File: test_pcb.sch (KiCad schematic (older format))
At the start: 22 parts, among them J1 Conn_01x04_Male, J11 Conn_01x20_Female, J8 Conn_01x20_Female, SW1 on/off, SW2 on/off

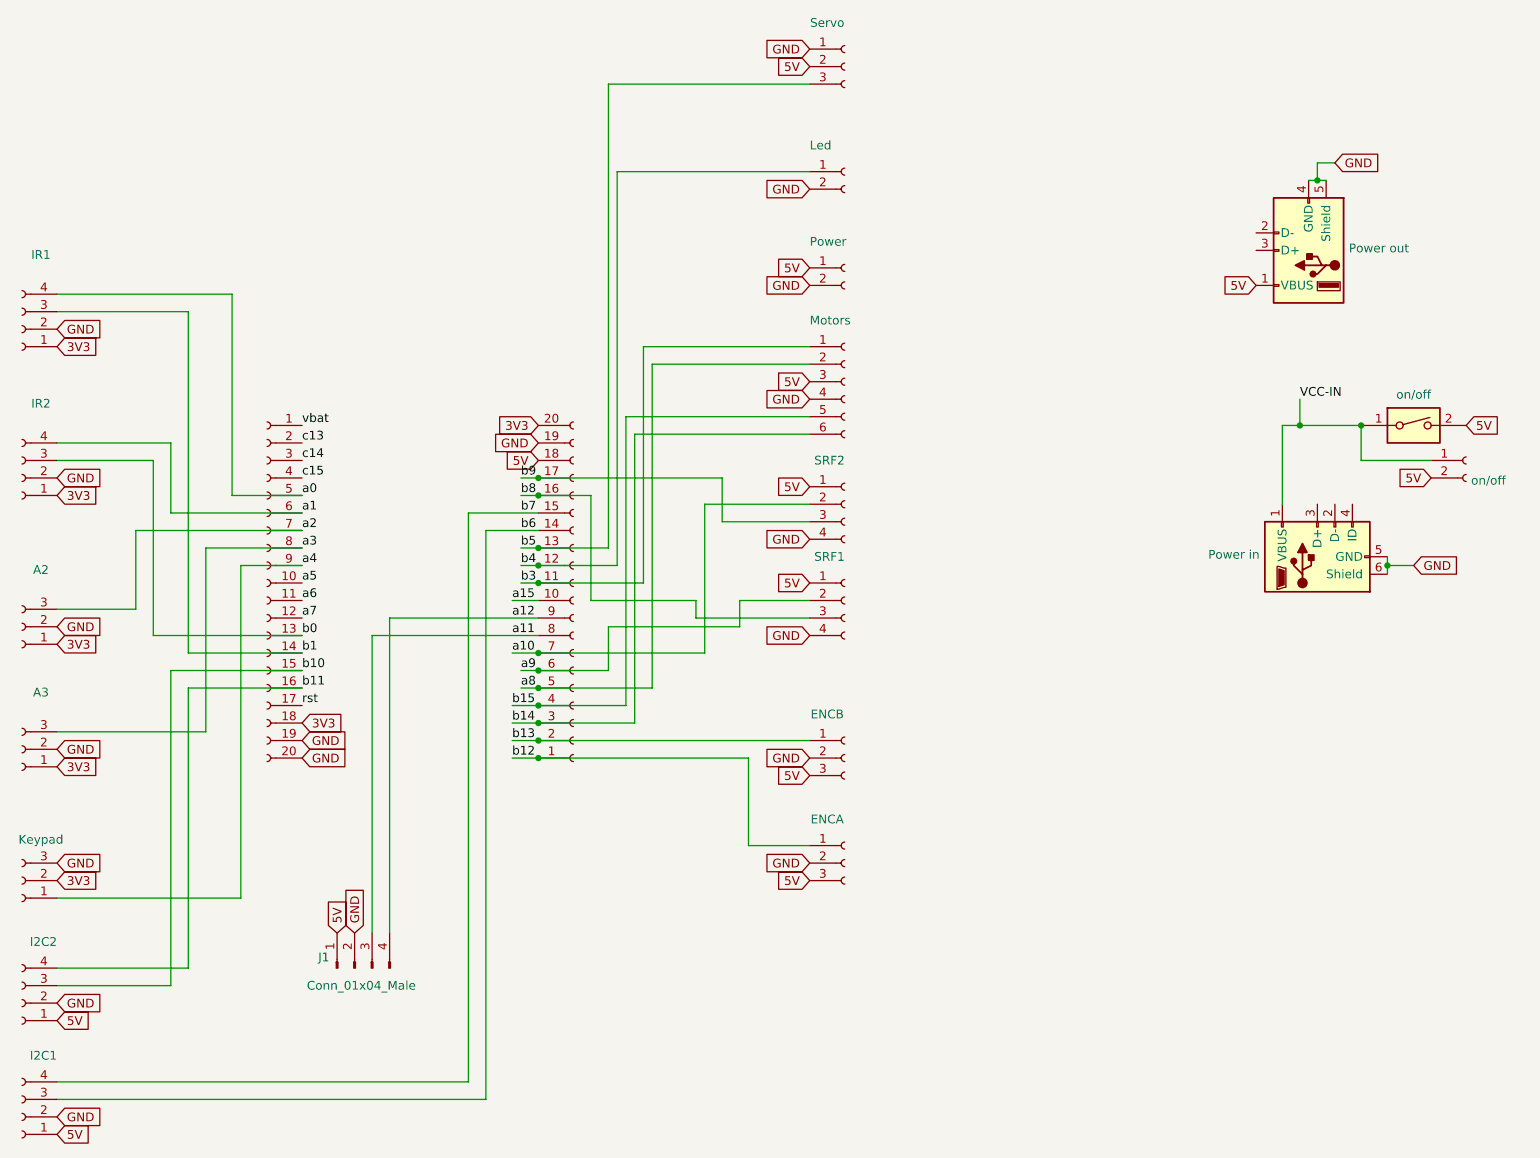
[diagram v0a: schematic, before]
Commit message: changes v2, ugly routing
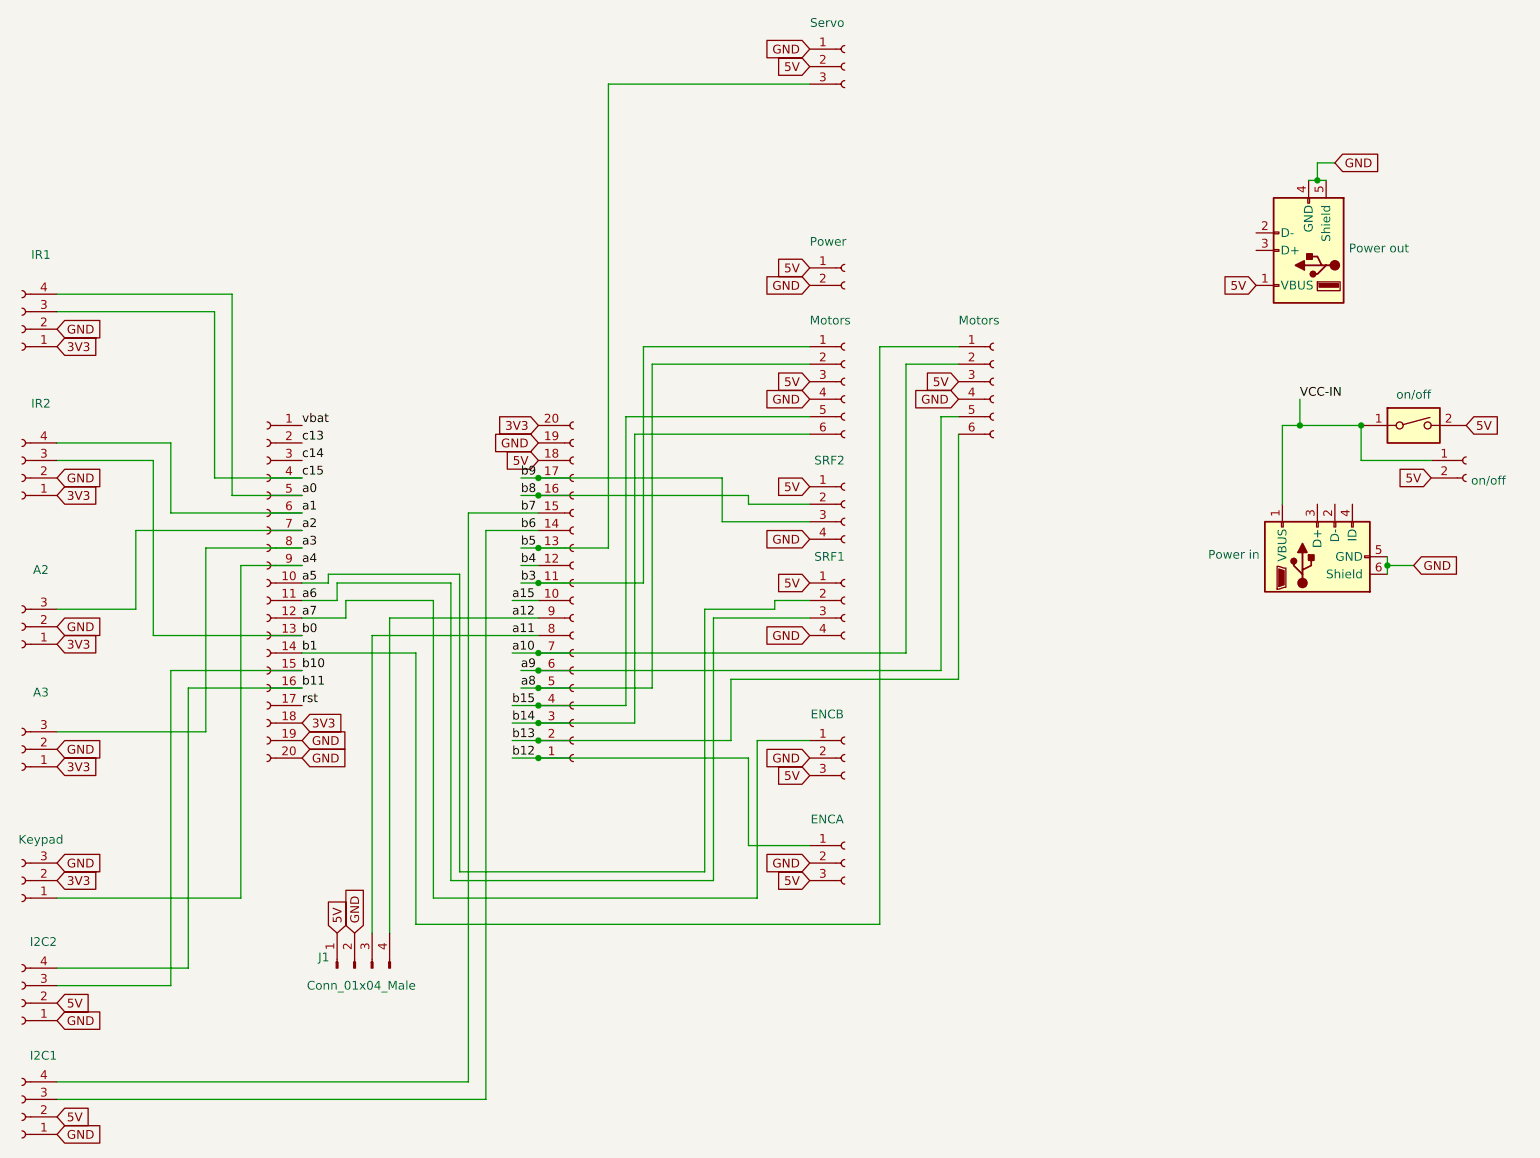
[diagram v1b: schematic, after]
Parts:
- removed led1: Led, Connector_PinSocket_2.54mm:PinSocket_1x02_P2.54mm_Vertical, symbol Connector:Conn_01x02_Female
- added mc2: Motors, Connector_PinSocket_2.54mm:PinSocket_1x06_P2.54mm_Vertical, symbol Connector:Conn_01x06_Female
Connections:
- net 5V: now also I2C1.2 (Pin_2), I2C2.2 (Pin_2), mc2.3 (Pin_3); no longer I2C1.1 (Pin_1), I2C2.1 (Pin_1)
- net GND: now also I2C1.1 (Pin_1), I2C2.1 (Pin_1), mc2.4 (Pin_4); no longer I2C1.2 (Pin_2), I2C2.2 (Pin_2)
- net a10: now also mc2.2 (Pin_2); no longer SRF2.2 (Pin_2)
- net a5: now also SRF1.2 (Pin_2)
- net a6: now also SRF1.3 (Pin_3)
- net a7: now also ENCB1.1 (Pin_1)
- net a9: now also mc2.5 (Pin_5); no longer SRF1.2 (Pin_2)
- net b1: now also mc2.1 (Pin_1); no longer IR1.3 (Pin_3)
- net b13: now also mc2.6 (Pin_6); no longer ENCB1.1 (Pin_1)
- net b8: now also SRF2.2 (Pin_2); no longer SRF1.3 (Pin_3)
- net c15: now also IR1.3 (Pin_3)
